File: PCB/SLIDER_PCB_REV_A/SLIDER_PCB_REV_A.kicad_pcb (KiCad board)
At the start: 2 copper layers, 5 parts, among them J1 V0, SW1 SW_Push

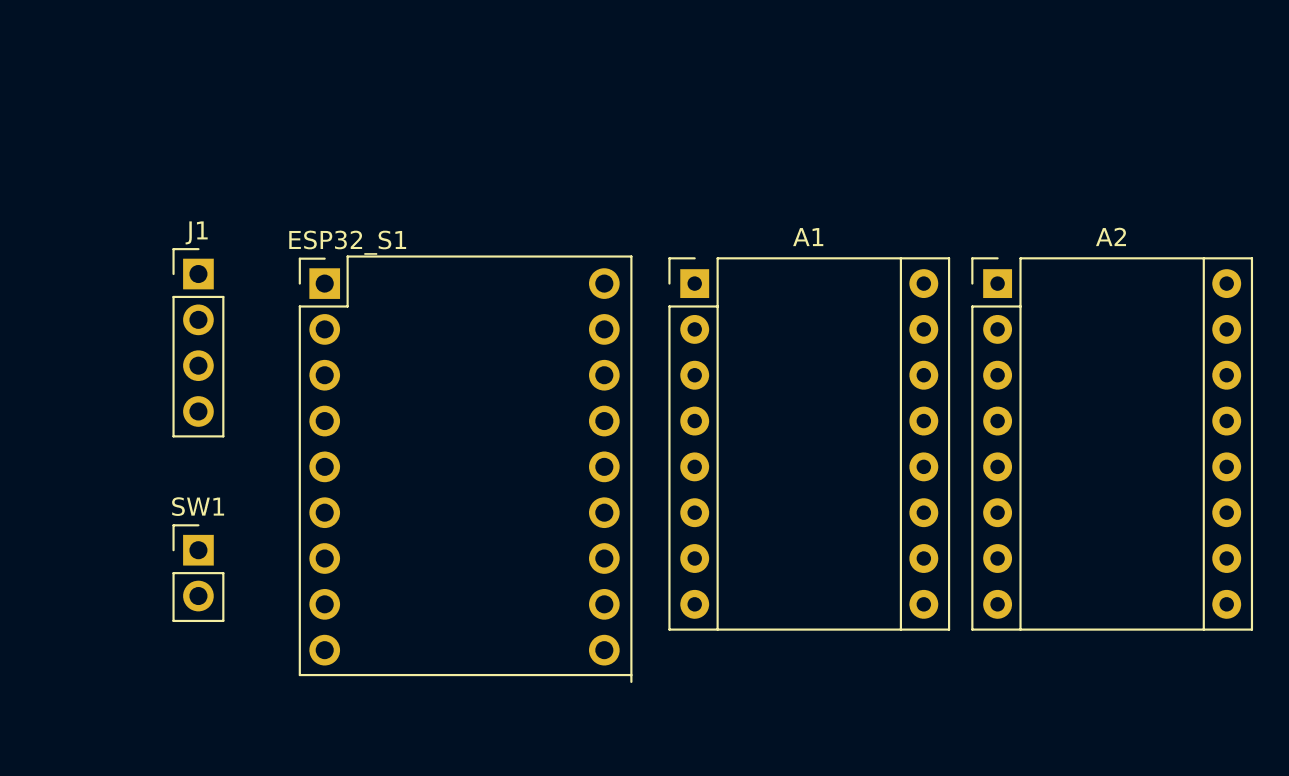
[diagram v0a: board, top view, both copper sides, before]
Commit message: 21h30 update : cad and PCB changes
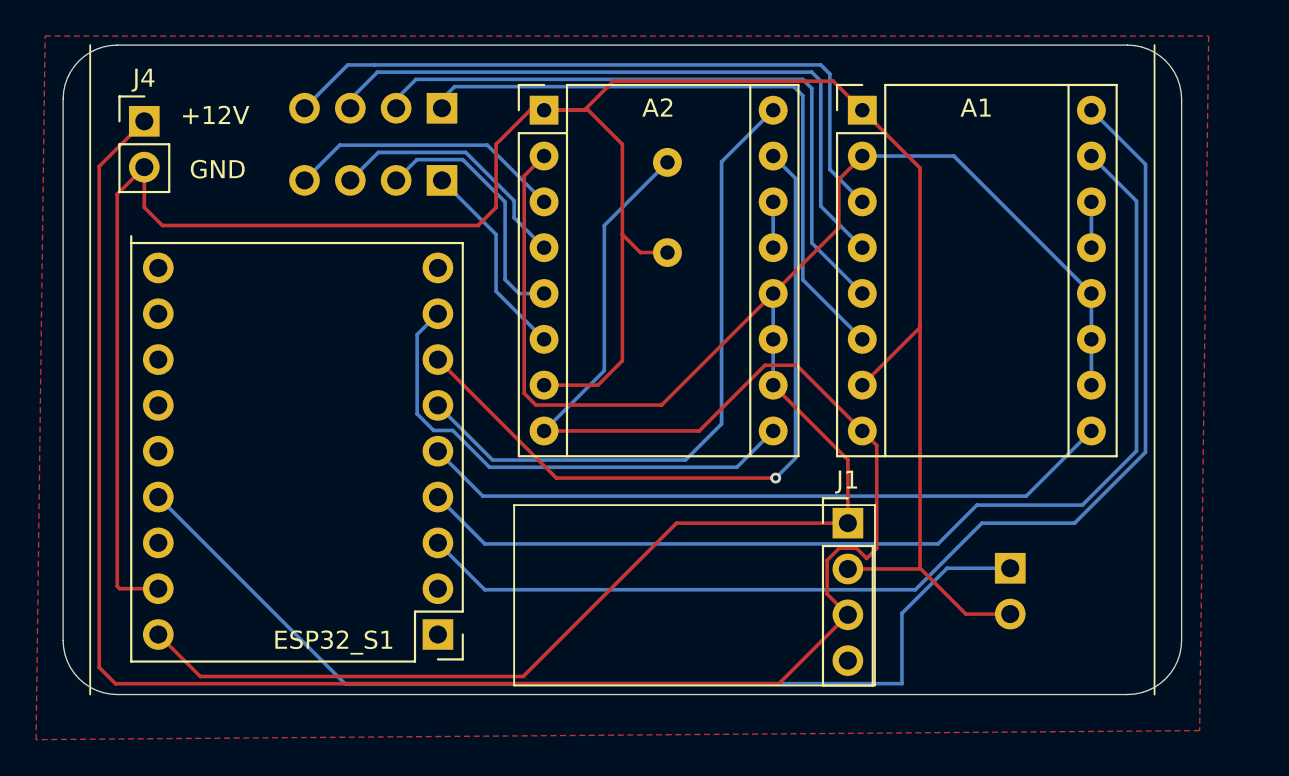
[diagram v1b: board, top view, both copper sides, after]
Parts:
- removed SW1: SW_Push, Connector_PinHeader_2.54mm:PinHeader_1x02_P2.54mm_Vertical
- added C2: C_Polarized, Capacitor_THT:C_Disc_D5.0mm_W2.5mm_P5.00mm, B.Cu at (105.5, 68.5)
- added J2: V0, Connector_PinHeader_2.54mm:PinHeader_1x04_P2.54mm_Vertical, B.Cu at (93.0, 65.5)
- added J3: V0, Connector_PinHeader_2.54mm:PinHeader_1x04_P2.54mm_Vertical, B.Cu at (93.0, 69.5)
- added J4: Conn_01x02_Pin, Connector_PinHeader_2.54mm:PinHeader_1x02_P2.54mm_Vertical, F.Cu at (76.5, 66.2)
- added J5: Conn_01x02_Pin, Connector_PinHeader_2.54mm:PinHeader_1x02_P2.54mm_Vertical, B.Cu at (124.5, 91.0)
- A1, A2: footprint Module:Pololu_Breakout-16_15.2x20.3mm -> ESP32-S3:Pololu_Breakout-16_15.2x20.3mm
- moved J1 38.6 mm to (115.5, 88.5)
- moved A2 26.9 mm to (98.7, 65.6)
- moved ESP32_S1 20.4 mm to (92.8, 94.7), turned to 180 degrees
- moved A1 13.4 mm to (116.3, 65.6)
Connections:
- A1 pad 1: unconnected-(A1-GND-Pad1) -> GND
- A1 pad 10: unconnected-(A1-MS1-Pad10) -> VDD
- A1 pad 11: unconnected-(A1-MS2-Pad11) -> VDD
- A1 pad 12: unconnected-(A1-MS3-Pad12) -> VDD
- A1 pad 13: unconnected-(A1-~{RESET}-Pad13) -> Net-(A1-~{RESET})
- A1 pad 14: unconnected-(A1-~{SLEEP}-Pad14) -> Net-(A1-~{RESET})
- A1 pad 15: unconnected-(A1-STEP-Pad15) -> Net-(A1-STEP)
- A1 pad 16: unconnected-(A1-DIR-Pad16) -> Net-(A1-DIR)
- A1 pad 2: unconnected-(A1-VDD-Pad2) -> VDD
- A1 pad 3: unconnected-(A1-1B-Pad3) -> Net-(A1-1B)
- A1 pad 4: unconnected-(A1-1A-Pad4) -> Net-(A1-1A)
- A1 pad 5: unconnected-(A1-2A-Pad5) -> Net-(A1-2A)
- A1 pad 6: unconnected-(A1-2B-Pad6) -> Net-(A1-2B)
- A1 pad 7: unconnected-(A1-GND-Pad7) -> GND
- A1 pad 8: unconnected-(A1-VMOT-Pad8) -> +12V
- A1 pad 9: unconnected-(A1-~{ENABLE}-Pad9) -> Net-(A1-~{ENABLE})
- A2 pad 1: unconnected-(A2-GND-Pad1) -> GND
- A2 pad 10: unconnected-(A2-MS1-Pad10) -> VDD
- A2 pad 11: unconnected-(A2-MS2-Pad11) -> VDD
- A2 pad 12: unconnected-(A2-MS3-Pad12) -> VDD
- A2 pad 13: unconnected-(A2-~{RESET}-Pad13) -> Net-(A2-~{RESET})
- A2 pad 14: unconnected-(A2-~{SLEEP}-Pad14) -> Net-(A2-~{RESET})
- A2 pad 15: unconnected-(A2-STEP-Pad15) -> Net-(A2-STEP)
- A2 pad 16: unconnected-(A2-DIR-Pad16) -> Net-(A2-DIR)
- A2 pad 2: unconnected-(A2-VDD-Pad2) -> VDD
- A2 pad 3: unconnected-(A2-1B-Pad3) -> Net-(A2-1B)
- A2 pad 4: unconnected-(A2-1A-Pad4) -> Net-(A2-1A)
- A2 pad 5: unconnected-(A2-2A-Pad5) -> Net-(A2-2A)
- A2 pad 6: unconnected-(A2-2B-Pad6) -> Net-(A2-2B)
- A2 pad 7: unconnected-(A2-GND-Pad7) -> GND
- A2 pad 8: unconnected-(A2-VMOT-Pad8) -> +12V
- A2 pad 9: unconnected-(A2-~{ENABLE}-Pad9) -> Net-(A2-~{ENABLE})
- ESP32_S1 pad 1: (no net) -> unconnected-(ESP32_S1-TX-Pad1)
- ESP32_S1 pad 10: (no net) -> unconnected-(ESP32_S1-12-Pad10)
- ESP32_S1 pad 11: (no net) -> Net-(A2-DIR)
- ESP32_S1 pad 12: (no net) -> unconnected-(ESP32_S1-11-Pad12)
- ESP32_S1 pad 13: (no net) -> Net-(A2-STEP)
- ESP32_S1 pad 14: (no net) -> unconnected-(ESP32_S1-10-Pad14)
- ESP32_S1 pad 15: (no net) -> Net-(A2-~{ENABLE})
- ESP32_S1 pad 16: (no net) -> unconnected-(ESP32_S1-9-Pad16)
- ESP32_S1 pad 17: (no net) -> unconnected-(ESP32_S1-7-Pad17)
- ESP32_S1 pad 18: (no net) -> unconnected-(ESP32_S1-8-Pad18)
- ESP32_S1 pad 2: (no net) -> VDD
- ESP32_S1 pad 3: (no net) -> unconnected-(ESP32_S1-RX-Pad3)
- ESP32_S1 pad 4: (no net) -> GND
- ESP32_S1 pad 5: (no net) -> Net-(A1-DIR)
- ESP32_S1 pad 6: (no net) -> unconnected-(ESP32_S1-3.3V(OUT)-Pad6)
- ESP32_S1 pad 7: (no net) -> Net-(A1-STEP)
- ESP32_S1 pad 8: (no net) -> Net-(ESP32_S1-13)
- ESP32_S1 pad 9: (no net) -> Net-(A1-~{ENABLE})
- J1 pad 1: unconnected-(J1-Pin_1-Pad1) -> VDD
- J1 pad 2: unconnected-(J1-Pin_2-Pad2) -> GND
- J1 pad 3: unconnected-(J1-Pin_3-Pad3) -> +12V
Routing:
- net GND: track 0.00 -> 141.1 mm
- net +12V: track 0.00 -> 127.0 mm
- net VDD: track 0.00 -> 118.0 mm
- net Net-(A1-DIR): track 0.00 -> 63.7 mm
- net Net-(A1-STEP): track 0.00 -> 59.3 mm
- net Net-(ESP32_S1-13): track 0.00 -> 56.4 mm
- net Net-(A2-STEP): track 0.00 -> 40.3 mm, vias 0 -> 1
- net Net-(A1-~{ENABLE}): track 0.00 -> 38.8 mm
- net Net-(A1-1B): track 0.00 -> 38.2 mm
- net Net-(A1-1A): track 0.00 -> 37.1 mm
- net Net-(A2-DIR): track 0.00 -> 36.4 mm
- net Net-(A1-2A): track 0.00 -> 36.2 mm
- net Net-(A1-2B): track 0.00 -> 35.4 mm
- net Net-(A2-~{ENABLE}): track 0.00 -> 27.8 mm
- net Net-(A2-1B): track 0.00 -> 15.4 mm
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- added copper zone on F.Cu, net GND
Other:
- board outline added: 62 x 36 mm
- board text added: "+12V"
- board text added: "100μF"
- board text added: "GND"
- board text added: "SIGNAL"
